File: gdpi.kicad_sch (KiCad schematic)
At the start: 22 parts, among them J7 HDMI_C_1.3, U1 ECP5U_12_CABGA256, U9 PCA9306DC1

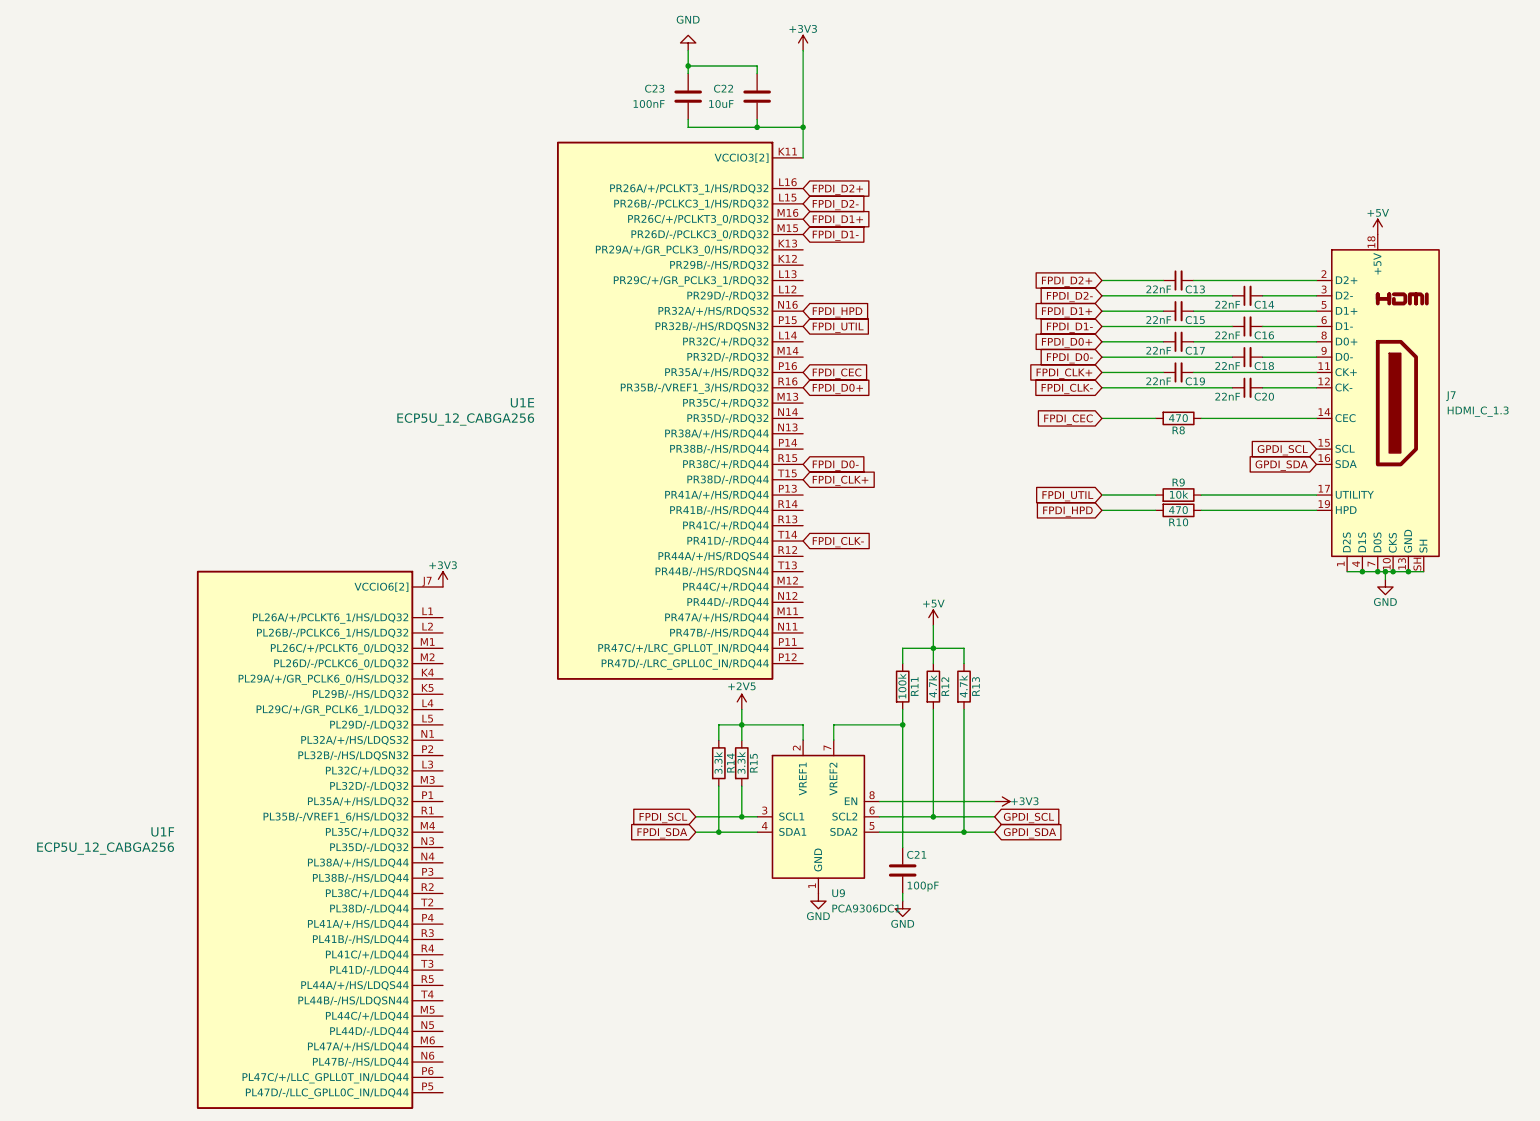
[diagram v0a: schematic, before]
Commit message: Stash
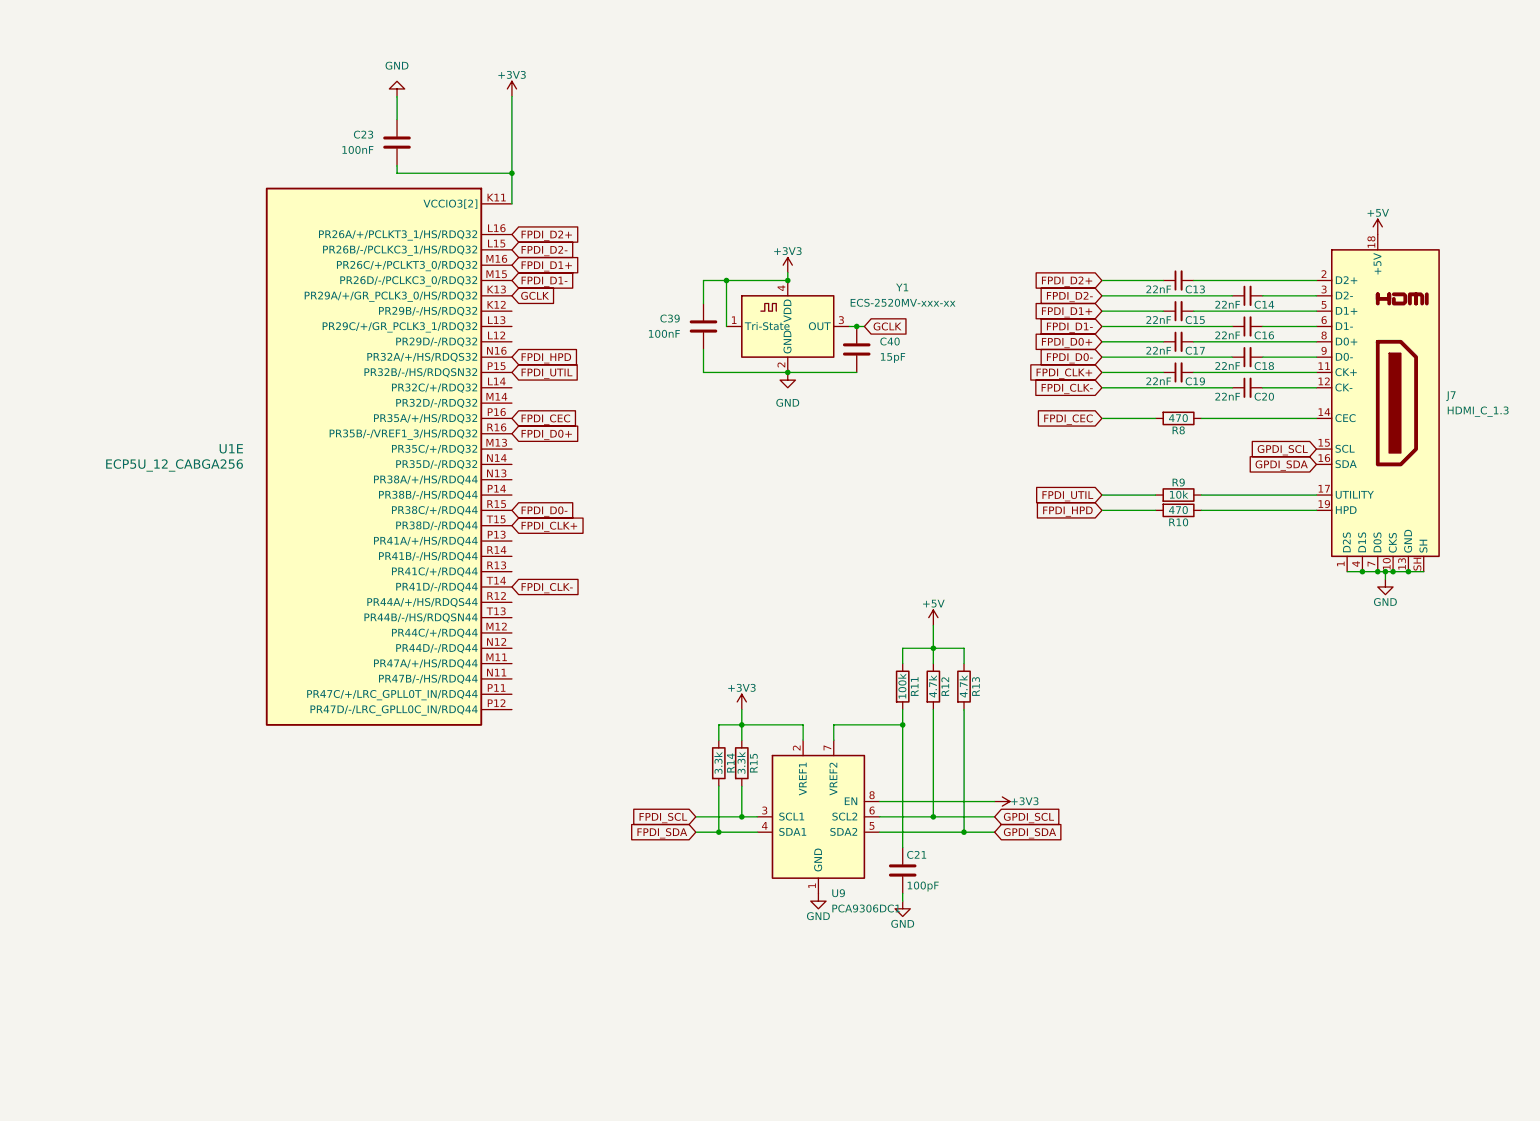
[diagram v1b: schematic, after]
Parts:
- removed C22: 10uF, Capacitor_SMD:C_0603_1608Metric, symbol Device:C
- removed unit 6 of U1
- added C39: 100nF, Capacitor_SMD:C_0402_1005Metric, symbol Device:C
- added C40: 15pF, Capacitor_SMD:C_0402_1005Metric, symbol Device:C
- added Y1: ECS-2520MV-xxx-xx, Crystal:Crystal_SMD_3225-4Pin_3.2x2.5mm, symbol Oscillator:ECS-2520MV-xxx-xx
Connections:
- net +2V5 is gone; now on net +3V3: R14.1, R15.1, U9.2 (VREF1)
- net +3V3: now also C39.1, Y1.1 (Tri-State), Y1.4 (VDD)
- net GND: now also C39.2, C40.2, Y1.2 (GND)
- net GCLK: now reaches U1.K13 (PR29A/+/GR_PCLK3_0/HS/RDQ32)
- net GCLK: now also C40.1, Y1.3 (OUT)
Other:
- moved on the sheet: C23, U1E

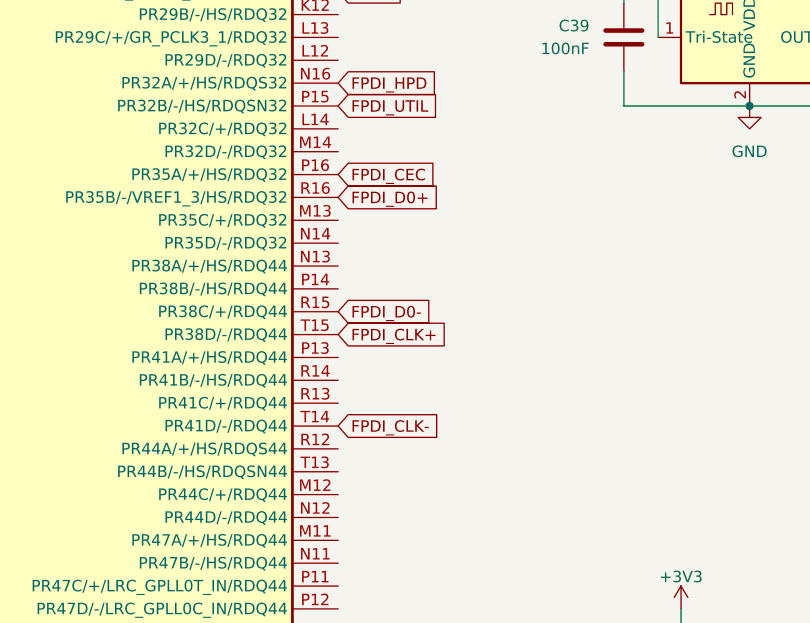
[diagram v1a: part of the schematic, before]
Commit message: Rev 1
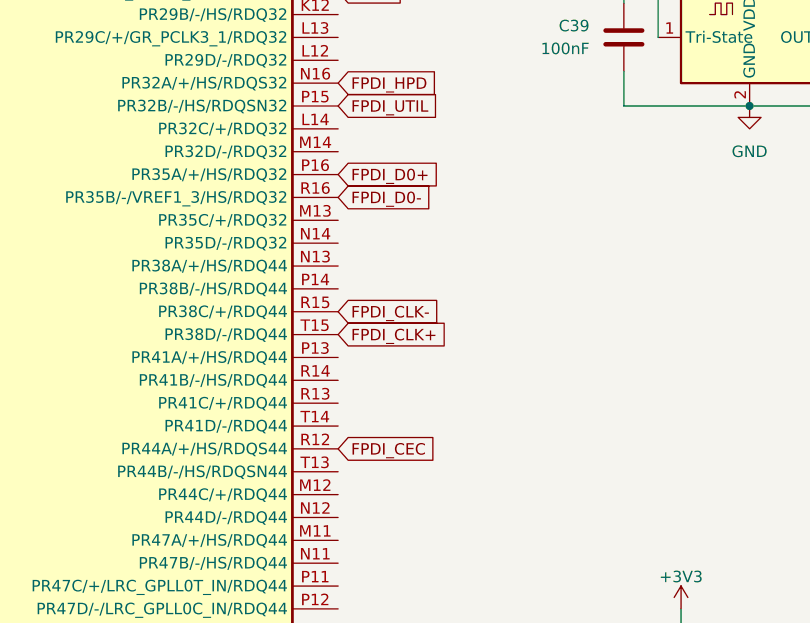
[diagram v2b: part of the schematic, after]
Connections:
- net FPDI_CEC: now also U1.R12 (PR44A/+/HS/RDQS44); no longer U1.P16 (PR35A/+/HS/RDQ32)
- net FPDI_CLK-: now also U1.R15 (PR38C/+/RDQ44); no longer U1.T14 (PR41D/-/RDQ44)
- net FPDI_D0+: now also U1.P16 (PR35A/+/HS/RDQ32); no longer U1.R16 (PR35B/-/VREF1_3/HS/RDQ32)
- net FPDI_D0-: now also U1.R16 (PR35B/-/VREF1_3/HS/RDQ32); no longer U1.R15 (PR38C/+/RDQ44)

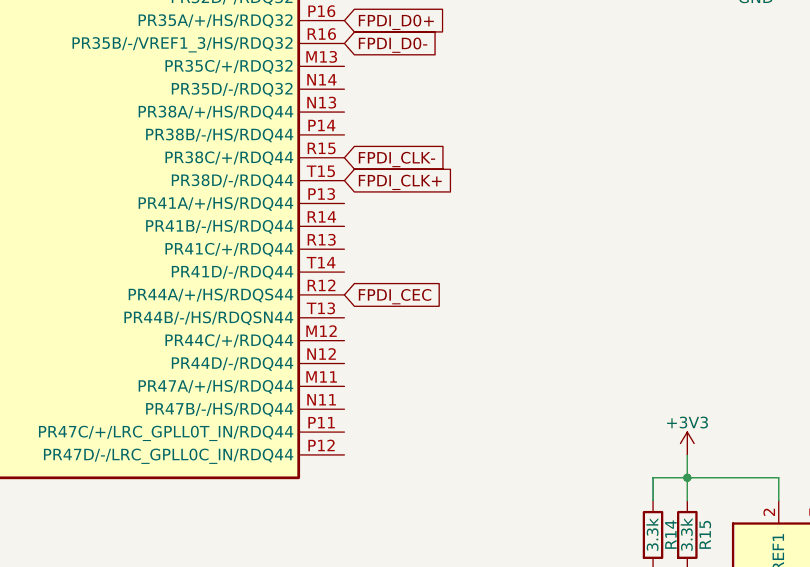
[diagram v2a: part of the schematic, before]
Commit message: No DRC Errors
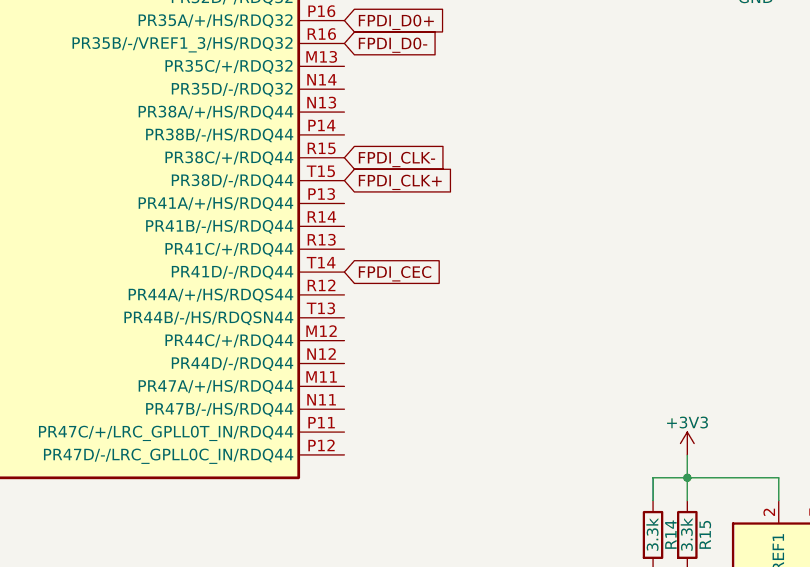
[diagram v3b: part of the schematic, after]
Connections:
- net FPDI_CEC: now also U1.T14 (PR41D/-/RDQ44); no longer U1.R12 (PR44A/+/HS/RDQS44)
